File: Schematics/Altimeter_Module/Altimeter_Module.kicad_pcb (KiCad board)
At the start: 4 copper layers, 69.5 x 60 mm, 104 parts, among them J1 Stack Male Edge Connector, J2 Main E-Match, J3 Drogue E-Match, J4 USB_B_Micro, J5 SWD_01x04_Pin, Q1 AO3400A, Q2 AO4406AL, Q3 AO3400A, Q4 AO3400A, Q5 AO4406AL, SW1 SW_STM_RESET, SW2 SW_STM_BOOT_MODE, U1 KX134-1211, U10 ACS70331EOLC, U12 AMS1117-3.3, U2 MS560702BA03-50, U3 W25Q128JVS, U4 LM66100DCKR, U5 LM66100DCKR, U6 STM32F103CBTx, U7 LM66100DCKR, U8 ISO1042BDWVR, U9 MPU-6050, Y1 X322516MMB4SI

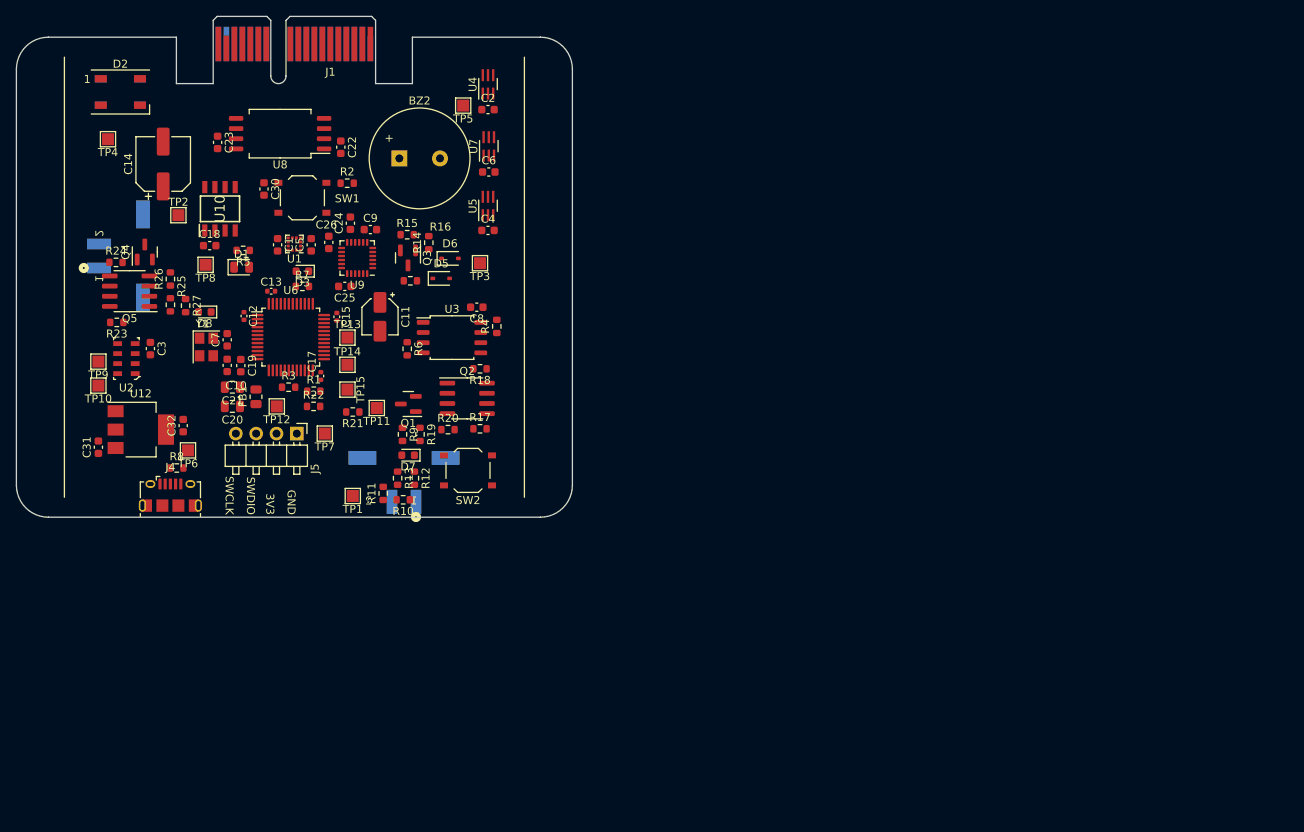
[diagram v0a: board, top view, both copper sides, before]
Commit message: progress 2:00 3/16
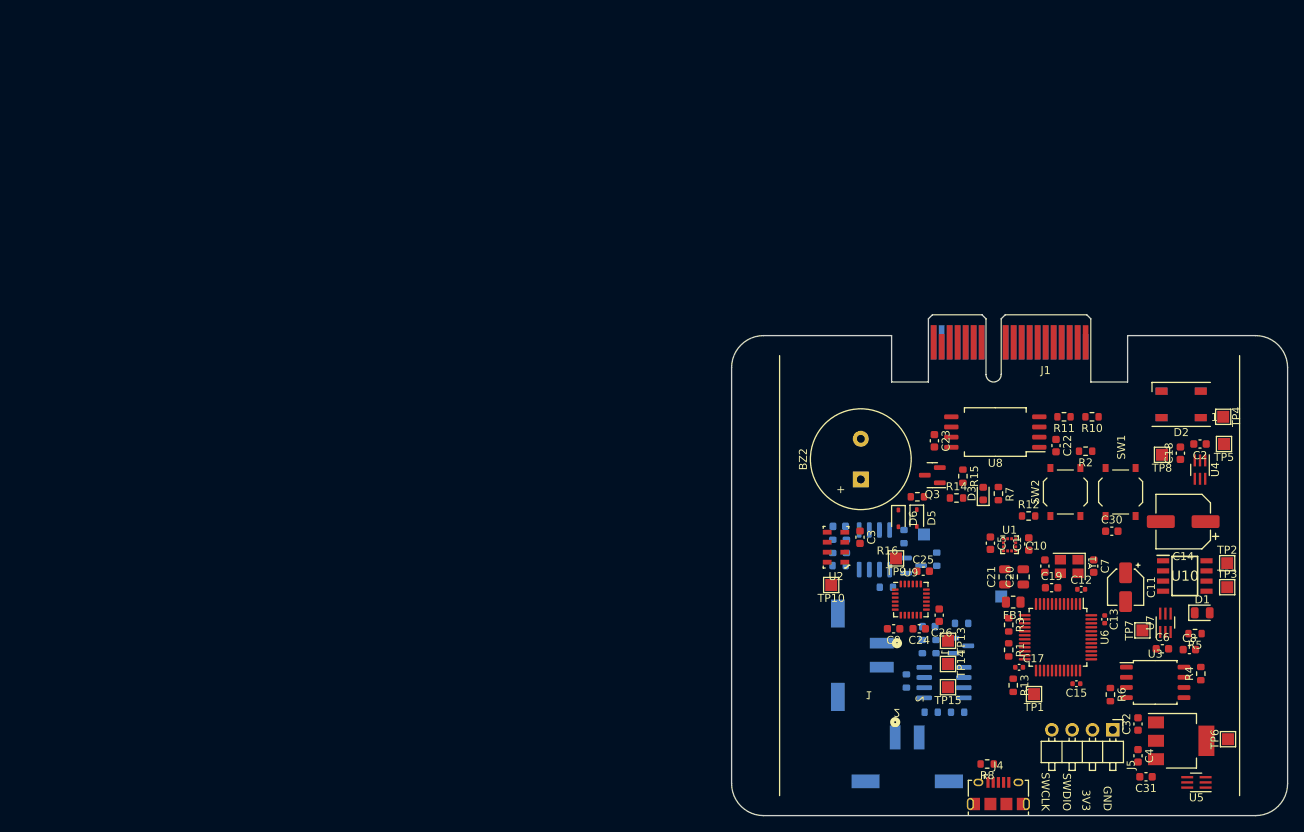
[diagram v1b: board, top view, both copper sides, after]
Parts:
- D7, D8, Q1, Q2, Q4, Q5, R17, R18, R19, R20, R21, R22, R23, R24, R25, R26, R27, R9, TP11, TP12: moved to B.Cu
- moved TP4 143.7 mm to (173.0, 67.6), turned to -90 degrees
- moved D2 138.2 mm to (167.8, 66.0), turned to 180 degrees
- moved D4 138.2 mm to (167.8, 66.0)
- moved TP2 138.1 mm to (173.5, 85.9)
- moved C31 137.3 mm to (163.3, 112.6), turned to 180 degrees
- moved U12 135.7 mm to (167.8, 108.1)
- moved C14 135.1 mm to (168.0, 80.7), turned to 180 degrees
- moved TP6 134.9 mm to (173.6, 107.9), turned to 90 degrees
- moved U10 129.0 mm to (168.2, 87.5), turned to 0 degrees
- moved R5 128.3 mm to (169.5, 94.7)
- moved D1 127.6 mm to (170.4, 92.1)
- moved C32 125.0 mm to (162.3, 106.0)
- moved C18 124.1 mm to (167.7, 72.2), turned to 90 degrees
- moved TP8 121.9 mm to (165.3, 72.3)
- moved C30 114.3 mm to (159.1, 81.9), turned to 0 degrees
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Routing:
- removed copper zone on In1.Cu, net GND
- removed copper zone on In2.Cu, net GND
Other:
- board text added: "Find way to place e-match parts"
